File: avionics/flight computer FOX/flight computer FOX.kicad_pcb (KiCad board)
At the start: 4 copper layers, 45.1 x 68.6 mm, 20 parts, among them J1 Screw_Terminal_01x02, U1 ESP32-DevKitC, U2 LM7805_TO220, U3 NRF24L01_Breakout

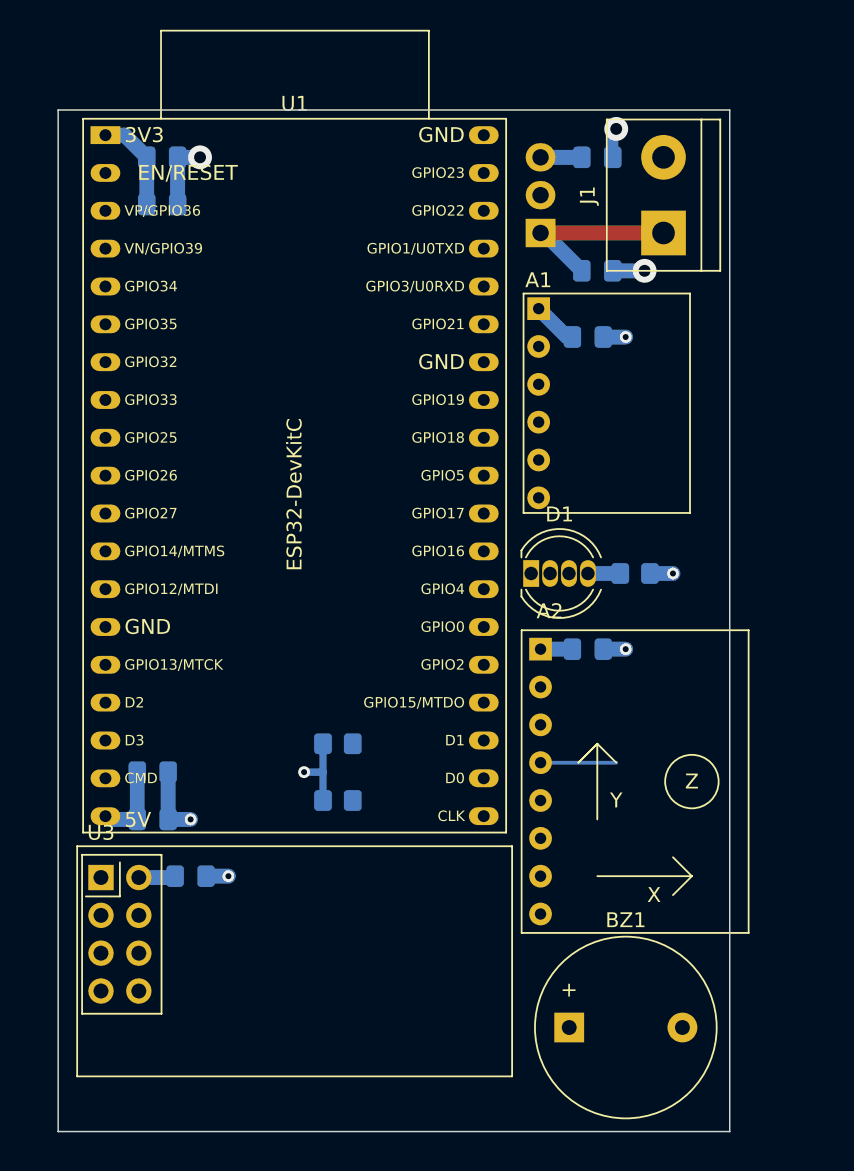
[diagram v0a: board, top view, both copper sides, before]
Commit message: more kicad
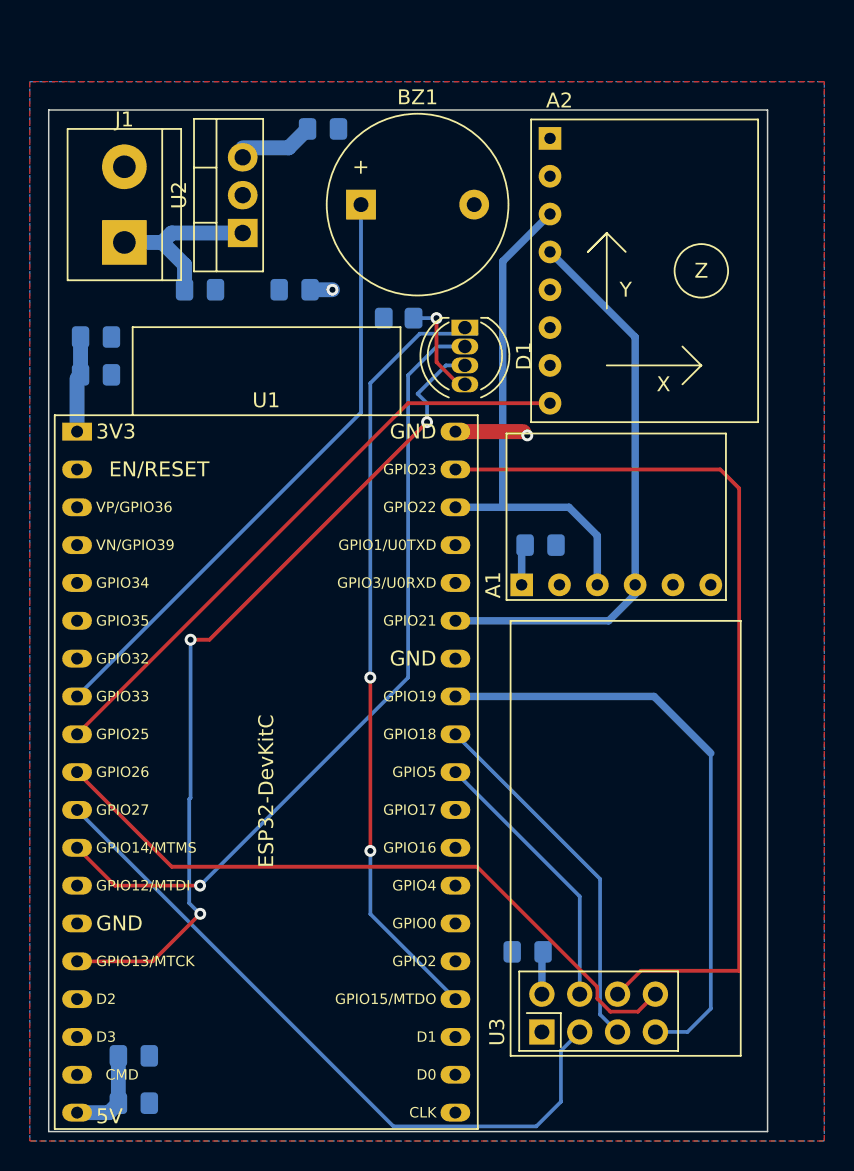
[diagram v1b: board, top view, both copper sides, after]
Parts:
- removed R2, R3: R10k, Resistor_SMD:R_0805_2012Metric_Pad1.20x1.40mm_HandSolder
- U2: moved to F.Cu
- moved C6 59.8 mm to (32.4, 86.4)
- moved BZ1 57.0 mm to (47.6, 26.0)
- moved C9 40.0 mm to (43.2, 31.8), turned to 180 degrees
- moved J1 36.2 mm to (31.8, 28.6)
- moved A2 34.3 mm to (60.3, 21.6)
- moved U3 31.4 mm to (59.8, 81.6), turned to 90 degrees
- moved C2 30.2 mm to (59.7, 48.9)
- moved C7 26.7 mm to (36.8, 31.8)
- moved R1 23.4 mm to (50.2, 33.7), turned to 0 degrees
- moved C5 20.7 mm to (58.8, 76.2), turned to 180 degrees
- moved U2 20.0 mm to (39.7, 27.9)
- moved U1 20.0 mm to (28.6, 41.3)
- moved A1 18.6 mm to (58.4, 51.6), turned to 90 degrees
- moved C8 18.5 mm to (45.1, 21.0)
- moved D1 17.1 mm to (54.6, 34.3), turned to -90 degrees
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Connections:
- U1 pad 12: unconnected-(U1-MTMS/GPIO14/ADC2_CH6-Pad12) -> greenled
- U1 pad 15: unconnected-(U1-MTCK/GPIO13/ADC2_CH4-Pad15) -> redled
- U1 pad 23: unconnected-(U1-*MTDO/GPIO15/ADC2_CH3-Pad23) -> blueled
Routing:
- net MOSI: track 0.00 -> 60.8 mm
- net redled: track 0.00 -> 56.4 mm, vias 0 -> 3
- net greenled: track 0.00 -> 54.0 mm, vias 0 -> 1
- net blueled: track 0.00 -> 53.2 mm, vias 0 -> 2
- net CE: track 0.00 -> 47.2 mm
- net INTNRF: track 0.00 -> 46.4 mm
- net INTMPU: track 0.00 -> 41.0 mm
- net buzzer: track 0.00 -> 40.9 mm
- net MISO: track 0.00 -> 40.2 mm
- net SCL: track 0.00 -> 34.6 mm
- net SDA: track 5.08 -> 38.2 mm
- net SCK: track 0.00 -> 24.5 mm
- net CS: track 0.13 -> 18.4 mm
- net GND: track 19.9 -> 4.57 mm, vias 8 -> 1
- net Net-(D1-K): track 2.17 -> 7.02 mm, vias 0 -> 1
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- added copper zone on F.Cu, net +5V
- added copper zone on B.Cu, net GND
- removed copper zone on In1.Cu, net +5V
- removed copper zone on In2.Cu, net GND
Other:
- board size 45.1 x 68.6 mm -> 48.3 x 68.6 mm
- copper layers 4 -> 2
